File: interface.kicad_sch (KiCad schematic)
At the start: 17 parts, among them J10 UART, J11 ST-Link, Q2 BSS138

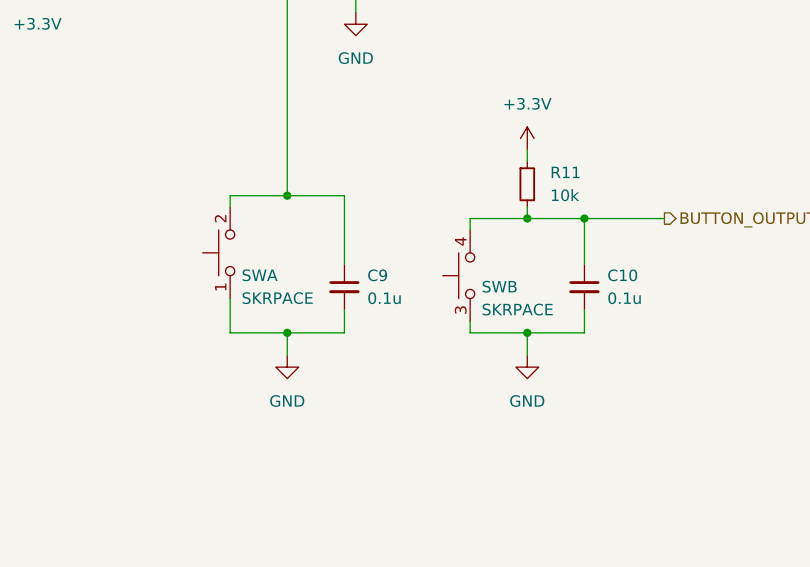
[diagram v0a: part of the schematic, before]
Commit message: update pcb
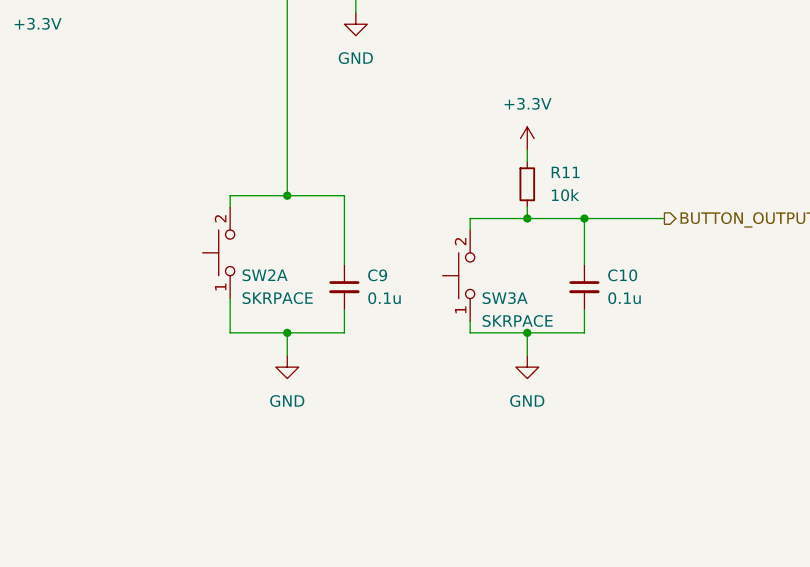
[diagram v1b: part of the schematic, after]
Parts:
- removed unit 2 of SW
- added SW3: SKRPACE, Button_Switch_SMD:SW_Push_1P1T_NO_Vertical_Wuerth_434133025816, symbol Switch:SW_Push_Dual_x2
- J10: footprint Connector_PinHeader_2.54mm:PinHeader_1x04_P2.54mm_Horizontal -> Connector_PinHeader_2.54mm:PinHeader_1x04_P2.54mm_Vertical
- J11: footprint Connector_JST:JST_SH_BM04B-SRSS-TB_1x04-1MP_P1.00mm_Vertical -> Connector_JST:JST_SH_SM04B-SRSS-TB_1x04-1MP_P1.00mm_Horizontal
- renumbered SW to SW2
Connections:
- net BUTTON_OUTPUT: now also SW3.2 (D)
- net GND: now also SW3.1 (C)
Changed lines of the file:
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@@
     (pin "2")
-  )
-  (symbol (lib_id "Switch:SW_Push_Dual_x2") (at 173.99 97.79 90) (unit 2)
-    (in_bom yes) (on_board yes)
-    (property "Reference" "SW" (id 0) (at 175.26 99.0599 90)
-      (effects (font (size 1.27 1.27)) (justify right))
-    )
-    (property "Value" "SKRPACE" (id 1) (at 175.26 101.5999 90)
-      (effects (font (size 1.27 1.27)) (justify right))
-    )
-    (property "Footprint" "Button_Switch_SMD:SW_Push_1P1T_NO_Vertical_Wuerth_434133025816" (id 2) (at 168.91 97.79 0)
-      (effects (font (size 1.27 1.27)) hide)
-    )
-    (property "Datasheet" "~" (id 3) (at 168.91 97.79 0)
-      (effects (font (size 1.27 1.27)) hide)
-    )
-    (pin "1")
-    (pin "2")
-    (pin "3")
-    (pin "4")
   )
   (symbol (lib_id "Device:LED") (at 82.55 60.96 90) (unit 1)
@@
   (symbol (lib_id "Switch:SW_Push_Dual_x2") (at 147.32 95.25 90) (unit 1)
     (in_bom yes) (on_board yes)
-    (property "Reference" "SW" (id 0) (at 148.59 97.7899 90)
+    (property "Reference" "SW2" (id 0) (at 148.59 97.7899 90)
       (effects (font (size 1.27 1.27)) (justify right))
     )
@@
       (effects (font (size 1.27 1.27)) (justify left))
     )
-    (property "Footprint" "Connector_JST:JST_SH_BM04B-SRSS-TB_1x04-1MP_P1.00mm_Vertical" (id 2) (at 168.91 59.69 0)
+    (property "Footprint" "Connector_JST:JST_SH_SM04B-SRSS-TB_1x04-1MP_P1.00mm_Horizontal" (id 2) (at 168.91 59.69 0)
       (effects (font (size 1.27 1.27)) hide)
     )
     (property "Datasheet" "~" (id 3) (at 168.91 59.69 0)
+      (effects (font (size 1.27 1.27)) hide)
+    )
+    (pin "1")
+    (pin "2")
+    (pin "3")
+    (pin "4")
+  )
+  (symbol (lib_id "Switch:SW_Push_Dual_x2") (at 173.99 97.79 90) (unit 1)
+    (in_bom yes) (on_board yes)
+    (property "Reference" "SW3" (id 0) (at 175.26 100.3299 90)
+      (effects (font (size 1.27 1.27)) (justify right))
+    )
+    (property "Value" "SKRPACE" (id 1) (at 175.26 102.8699 90)
+      (effects (font (size 1.27 1.27)) (justify right))
+    )
+    (property "Footprint" "Button_Switch_SMD:SW_Push_1P1T_NO_Vertical_Wuerth_434133025816" (id 2) (at 168.91 97.79 0)
+      (effects (font (size 1.27 1.27)) hide)
+    )
+    (property "Datasheet" "~" (id 3) (at 168.91 97.79 0)
       (effects (font (size 1.27 1.27)) hide)
     )
@@
       (effects (font (size 1.27 1.27)) (justify left))
     )
-    (property "Footprint" "Connector_PinHeader_2.54mm:PinHeader_1x04_P2.54mm_Horizontal" (id 2) (at 128.27 59.69 0)
-      (effects (font (size 1.27 1.27)) hide)
-    )
+    (property "Footprint" "Connector_PinHeader_2.54mm:PinHeader_1x04_P2.54mm_Vertical" (id 2) (at 128.27 59.69 0)
+      (effects (font (size 1.27 1.27)) hide)
+    )
